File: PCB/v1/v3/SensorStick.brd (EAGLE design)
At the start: 76.2 x 44.5 mm, 56 parts, among them U1 TPD4F003DQDR, Y1 ECS-TXO-3225MV-400-TR

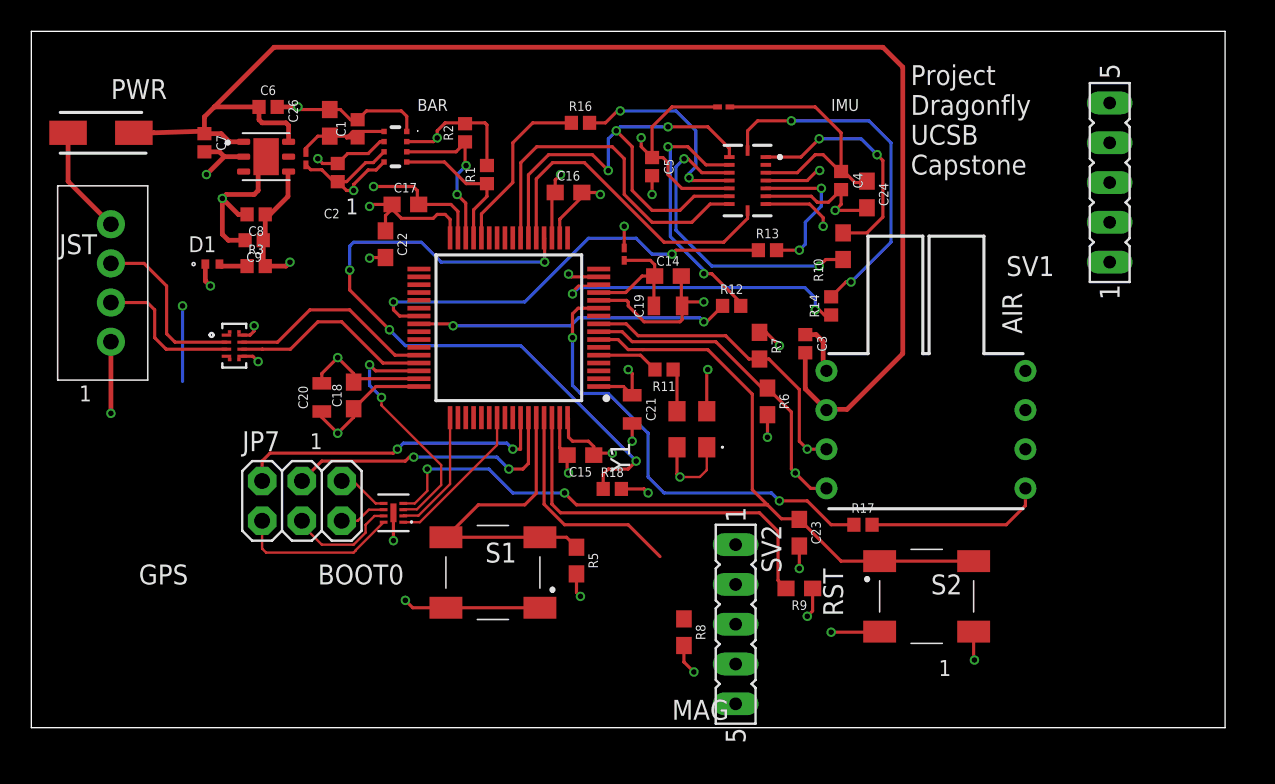
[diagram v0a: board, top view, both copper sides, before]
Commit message: Jesus - Cleaned up sch/layout, finished
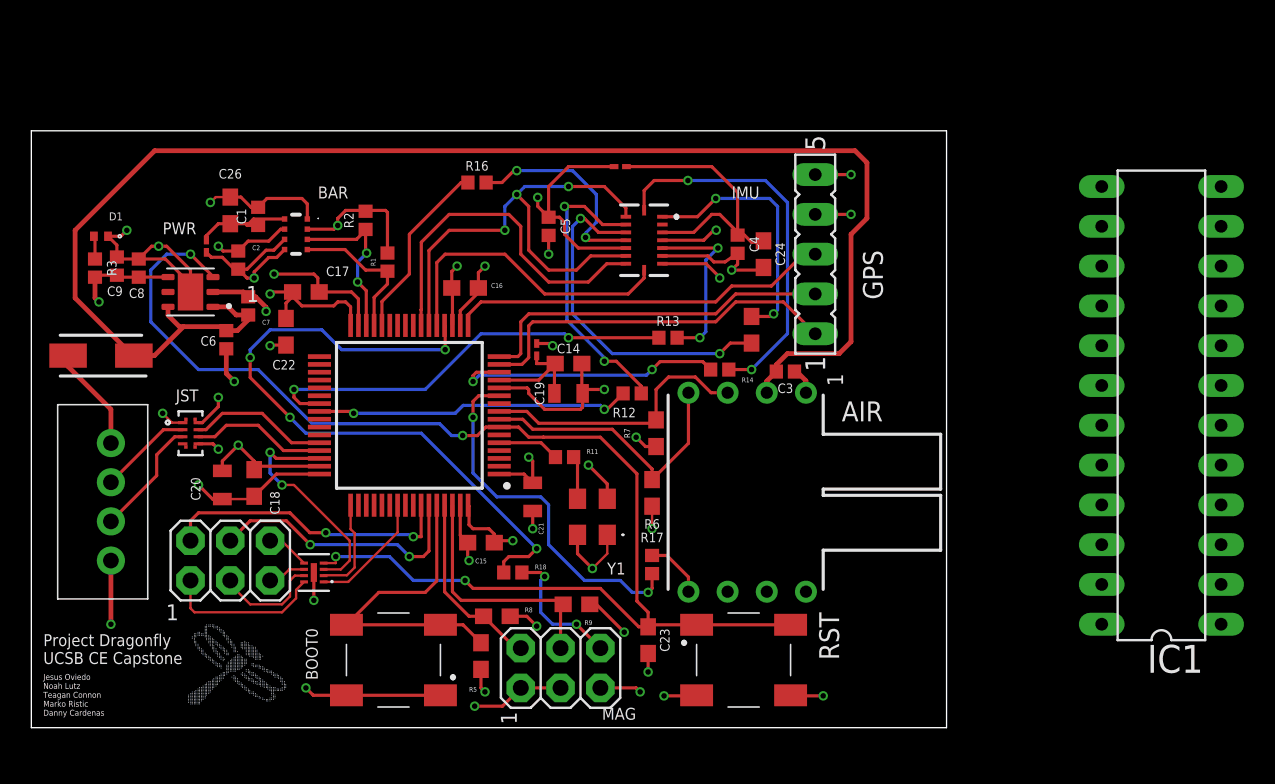
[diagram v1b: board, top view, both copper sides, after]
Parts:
- removed SV2: (no value), con-lsta:FE05-1
- added IC1: (no value), ic-package:DIL24-3
- added JP1: (no value), pinhead:2X03
- moved SV1 19.3 mm to (50.0, 30.2)
- moved C6 15.1 mm to (12.4, 24.8), turned to 270 degrees
- moved R9 14.3 mm to (34.8, 7.87)
- moved U$1 14.2 mm to (4.45, 23.7)
- moved JST_CONNECTION 14.0 mm to (5.08, 10.7)
- moved AIRSPEED 13.7 mm to (50.5, 13.1), turned to 180 degrees
- moved R17 13.7 mm to (39.6, 10.4), turned to 90 degrees
- moved S2 12.4 mm to (45.5, 4.32)
- moved R8 12.0 mm to (29.7, 7.11), turned to 0 degrees
- moved C23 11.8 mm to (39.4, 5.59)
- moved C7 10.8 mm to (13.8, 26.9), turned to 90 degrees
- moved R3 10.3 mm to (4.06, 29.3), turned to 270 degrees
- moved POWER_MODULE 9.89 mm to (10.2, 27.8), turned to 180 degrees
- moved R6 9.40 mm to (39.6, 15.0)
- moved C16 8.99 mm to (27.7, 28.1)
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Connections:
- net 3V3: now also JP1.1, JP1.3; no longer SV2.5
- net EXTI4: now also JP1.6; no longer SV2.1
- net GND: now also JP1.5; no longer SV2.4
- net I2C1_SCL: now also JP1.2; no longer SV2.3
- net I2C1_SDA: now also JP1.4; no longer SV2.2
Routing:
- net USART2_RX: track 0.00 -> 24.4 mm
- net USART2_TX: track 0.00 -> 23.0 mm
- net NRST: track 64.1 -> 86.1 mm, vias 3 -> 4
- net GPIO_EXTI1: track 2.00 -> 23.9 mm, vias 1 -> 0
- net I2C1_SDA: track 24.5 -> 15.8 mm
- net 3V3: track 95.0 -> 103.2 mm, vias 16 -> 19
- net EXTI3: track 11.4 -> 3.83 mm
- net EXTI4: track 1.81 -> 8.71 mm, vias 1 -> 2
- net GPIO_EXTI3: track 29.7 -> 23.5 mm
- net DN: track 11.2 -> 5.97 mm
- net USB_DP: track 13.1 -> 8.70 mm
- net USB_DN: track 13.3 -> 8.94 mm
- net GND: track 109.9 -> 114.2 mm, vias 25 -> 28
- net 5V: track 90.9 -> 94.9 mm
- net I2C3_SCL: track 20.8 -> 18.3 mm, vias 1 -> 0
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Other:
- board size 76.2 x 44.5 mm -> 58.4 x 38.1 mm
- board text added: "Jesus Oviedo Noah Lutz Teagan Connon Marko Ristic Danny Cardenas"
- board text added: "Project Dragonfly UCSB CE Capstone"
- board text added: "⠀⠀⠀⠀⠀⠀⢀⣀⣀⠀⠀⠀⠀⠀⠀⠀⠀⠀⠀⠀⠀⠀⠀⠀⠀⠀⠀⠀⠀⠀ ⠀⠀⠀⠀⠀⠀⣿⠉⠙⠻⣦⡀⠀⠀⠀⠀⠀⠀⠀⠀⠀⠀⠀⠀⠀⠀⠀⠀⠀⠀ ⠀⠀⢀⣶⠿⠶⣿⣄⠀⠀⠈⢿⣄⠀⠀⠀⠀⠀⠀⠀⠀⠀⠀⠀⠀⠀⠀⠀⠀⠀ ⠀⠀⠈⣧⠀⠀⠘⣿⣷⣄⠀⠀⢻⣦⠀⠀⣀⣄⡀⠀⠀⠀⠀⠀⠀⠀⠀⠀⠀⠀ ⠀⠀⠀⠘⣧⡀⠀⠘⣷⡙⢷⣄⠀⠹⣧⠀⢿⣿⣷⣦⡄⠀⠀⠀⠀⠀⠀⠀⠀⠀ ⠀⠀⠀⠀⠈⢿⣄⠀⠘⢷⡄⠹⣧⠀⠛⣂⠀⢸⣿⣿⣿⣄⠀⠀⠀⠀⠀⠀⠀⠀ ⠀⠀⠀⠀⠀⠀⠙⢷⣄⠈⠻⡦⠀⣠⣾⣿⣷⣤⠈⠙⠿⠿⠁⠀⠀⠀⠀⠀⠀⠀ ⠀⠀⠀⠀⠀⠀⠀⠀⠙⢷⣦⠀⣼⣿⣿⣿⣿⠟⠀⢶⣤⣄⡀⠀⠀⠀⠀⠀⠀⠀ ⠀⠀⠀⠀⠀⠀⠀⠀⠀⠀⠈⣀⣿⠿⠿⠛⢁⠰⣦⣀⠀⠉⠻⢶⣤⡀⠀⠀⠀⠀ ⠀⠀⠀⠀⠀⠀⠀⠀⢀⣤⣾⡟⠁⠠⣦⡀⠙⢷⣌⡛⢷⣄⠀⠀⠈⠻⢷⣄⠀⠀ ⠀⠀⠀⠀⠀⠀⣠⣶⣿⣿⠋⠀⠀⠀⠙⢷⣄⠀⠉⠻⢶⣽⣷⣄⠀⠀⠀⢻⣆⠀ ⠀⠀⠀⢀⣴⣾⣿⣿⠟⠁⠀⠀⠀⠀⠀⠀⠙⢷⣄⠀⠀⠈⠙⠻⣷⣶⣤⣴⠟⠀ ⠀⢠⣾⣿⣿⣿⡿⠋⠀⠀⠀⠀⠀⠀⠀⠀⠀⠀⠙⠻⣦⡀⠀⠀⠸⣧⠀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"
- board text removed: "Project Dragonfly UCSB Capstone"
